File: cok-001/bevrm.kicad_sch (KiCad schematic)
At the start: 11 parts, among them U6103 NCP5318FTR2G, U6104 iP2003APbF, U6105 iP2003APbF, U6106 iP2003APbF, U6107 TC7SG08FU

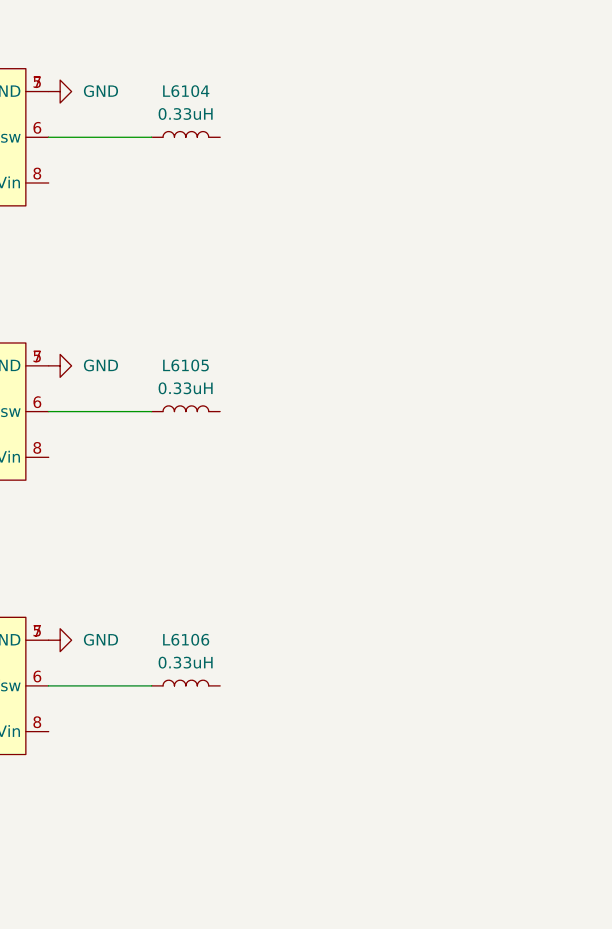
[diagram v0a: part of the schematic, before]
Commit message: chris proad
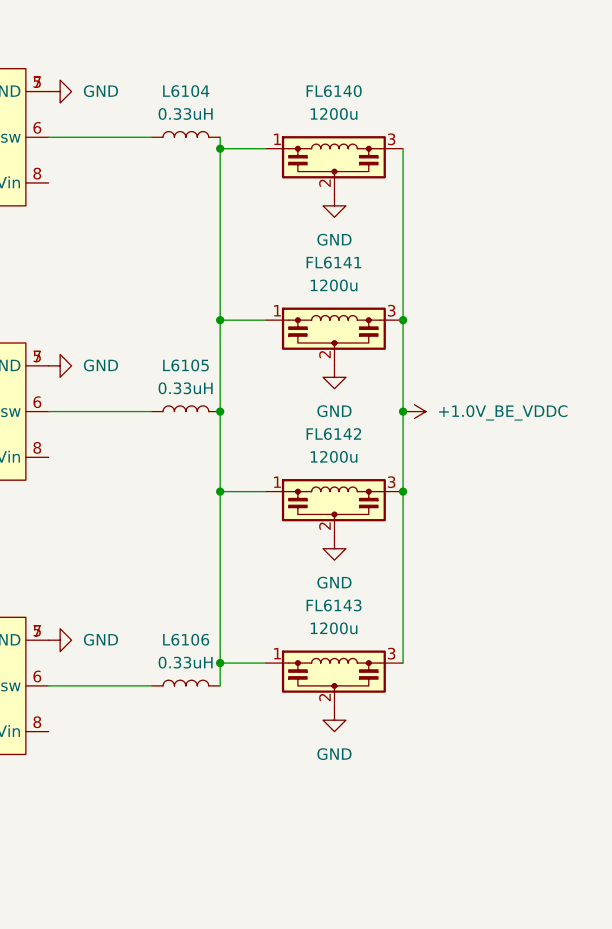
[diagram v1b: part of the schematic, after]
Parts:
- added FL6140, FL6141, FL6142, FL6143: 1200u, PS3:Proadlizer, symbol Device:Filter_EMI_CLC
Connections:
- net GND: now also FL6140.2, FL6141.2, FL6142.2, FL6143.2
- net at L6105.2: now also L6104.2, L6106.2, FL6140.1, FL6141.1, FL6142.1, FL6143.1
- new net +1.0V_BE_VDDC: FL6140.3, FL6141.3, FL6142.3, FL6143.3

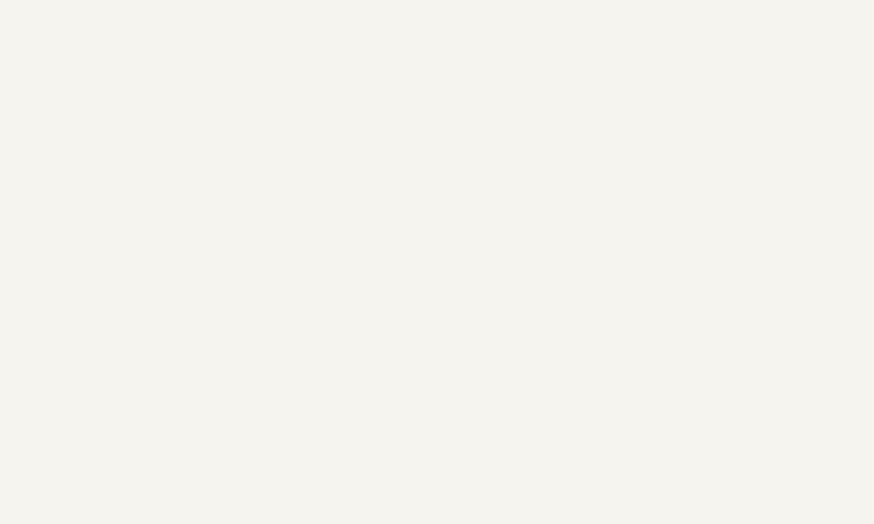
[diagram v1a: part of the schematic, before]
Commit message: temp sensor and clock
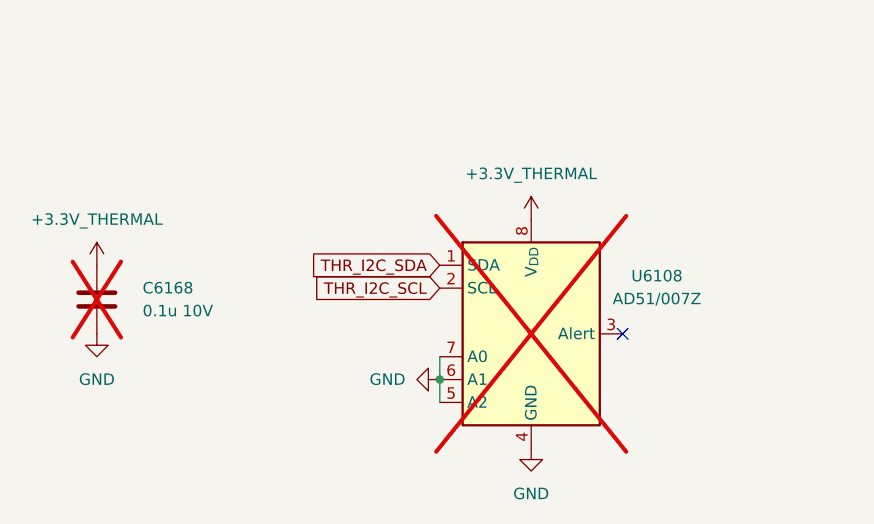
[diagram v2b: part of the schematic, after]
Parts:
- added C6168: 0.1u 10V, Capacitor_SMD:C_0402_1005Metric, symbol Device:C
- added U6108: AD51/007Z, Package_SO:MSOP-8_3x3mm_P0.65mm, symbol Sensor_Temperature:MCP9804_MSOP
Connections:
- net GND: now also C6168.2, U6108.4 (GND), U6108.5 (A2), U6108.6 (A1), U6108.7 (A0)
- new net +3.3V_THERMAL: C6168.1, U6108.8 (V_{DD})
- new net THR_I2C_SCL: U6108.2 (SCL)
- new net THR_I2C_SDA: U6108.1 (SDA)
- no-connect marks 0 -> 1

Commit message: msop
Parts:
- U6108: footprint Package_SO:MSOP-8_3x3mm_P0.65mm -> PS3:MSOP-8_2.9x4mm_P0.65mm
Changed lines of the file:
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@@
 			)
 		)
-		(property "Footprint" "Package_SO:MSOP-8_3x3mm_P0.65mm"
+		(property "Footprint" "PS3:MSOP-8_2.9x4mm_P0.65mm"
 			(at 43.18 176.53 0)
 			(effects

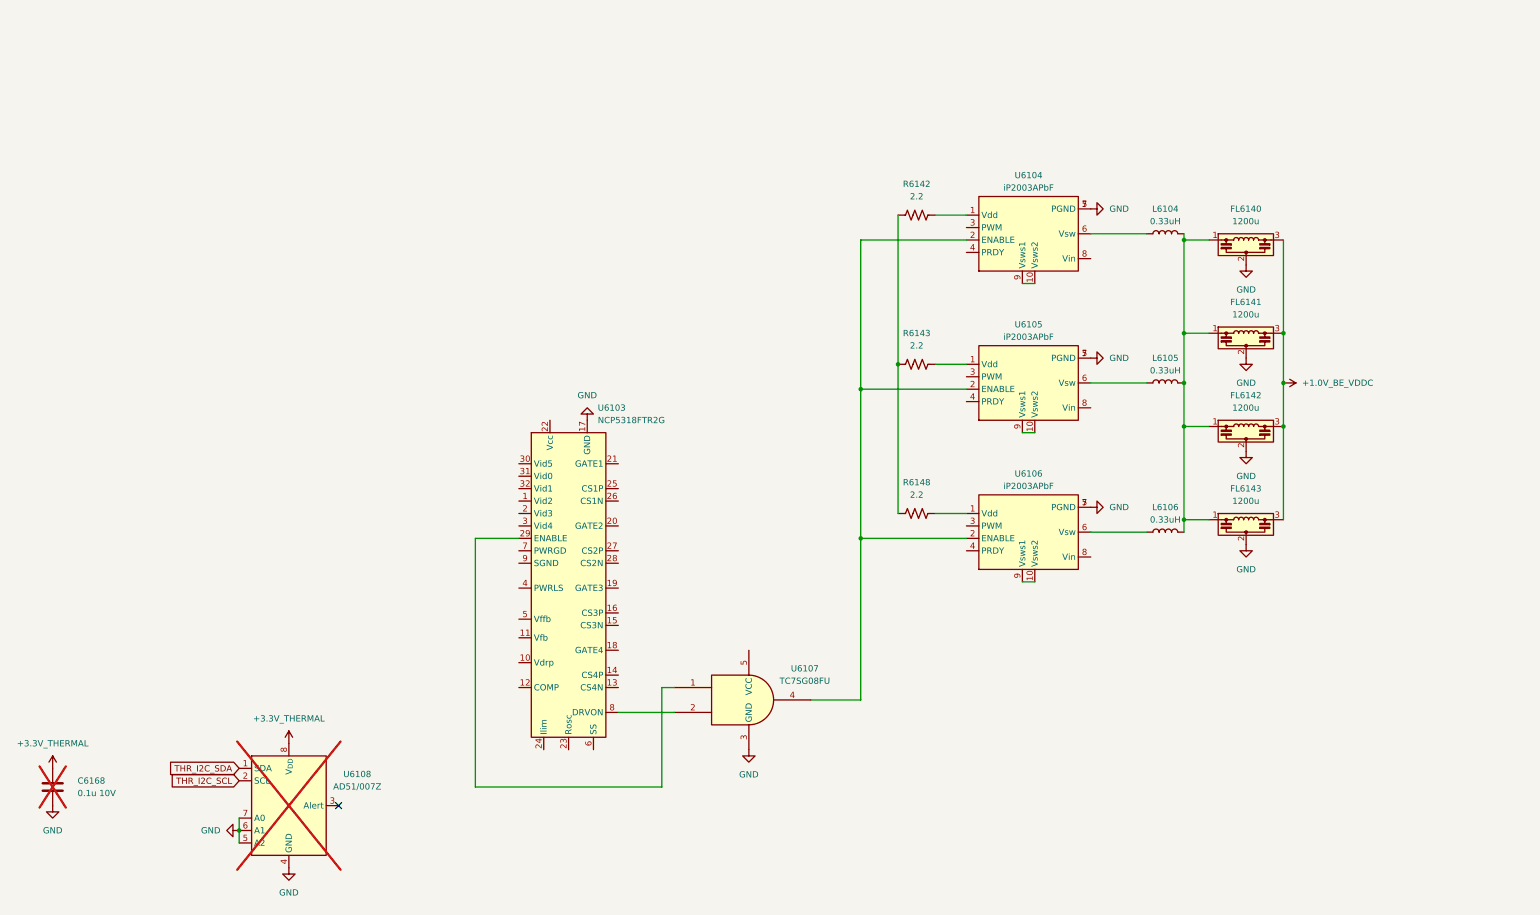
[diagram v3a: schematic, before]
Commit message: current sense
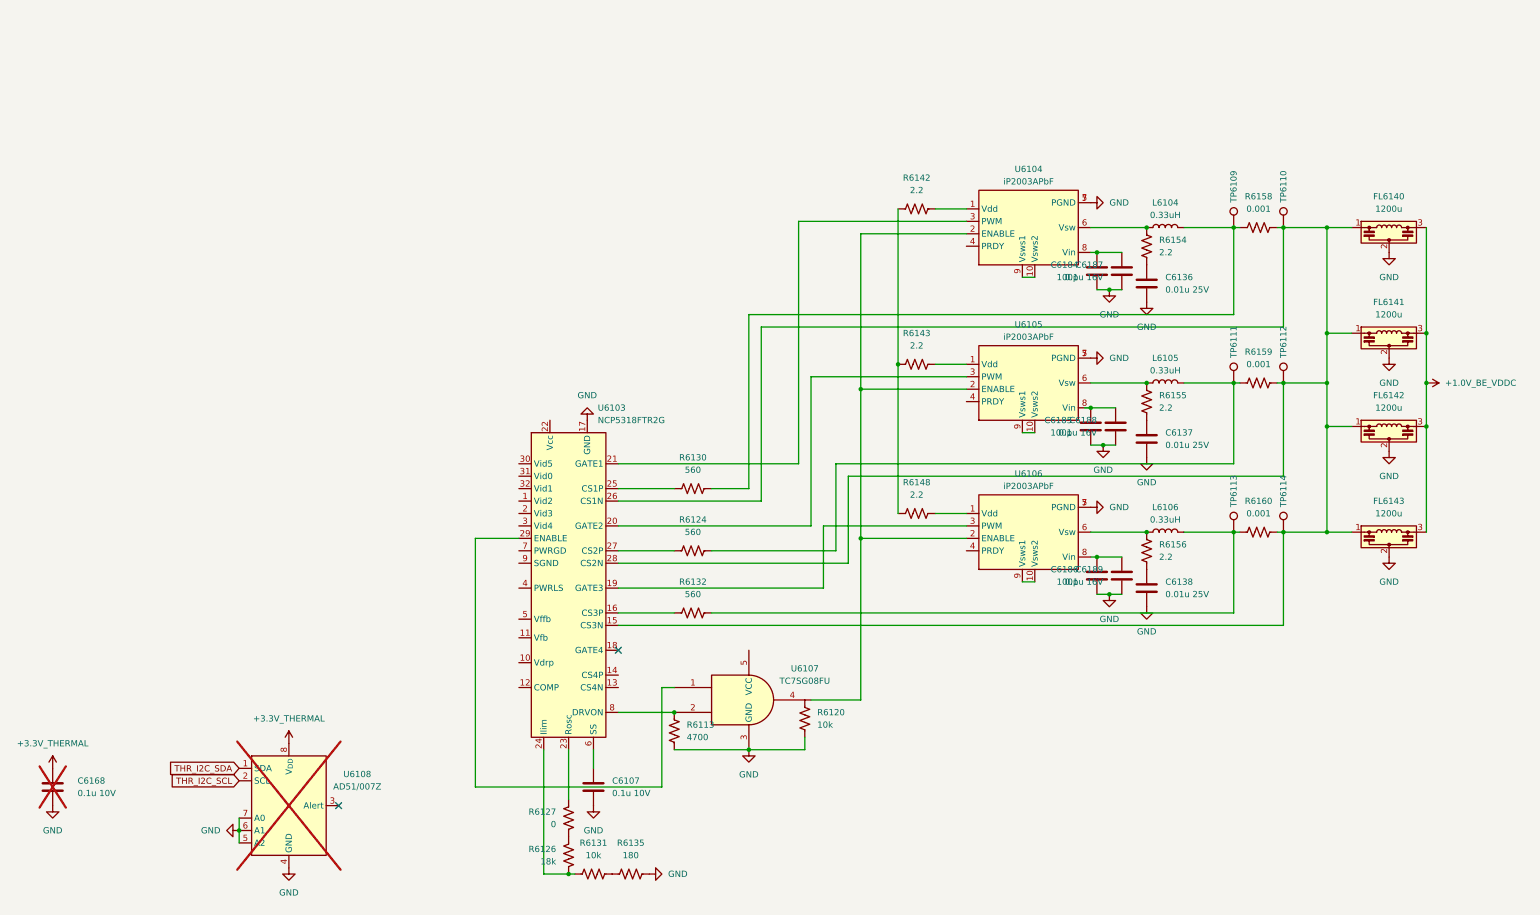
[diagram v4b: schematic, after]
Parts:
- added C6107: 0.1u 10V, Capacitor_SMD:C_0402_1005Metric, symbol Device:C
- added C6136, C6137, C6138: 0.01u 25V, Capacitor_SMD:C_0402_1005Metric, symbol Device:C
- added C6184, C6185, C6186: 100p, Capacitor_SMD:C_0402_1005Metric, symbol Device:C
- added C6187, C6188, C6189: 0.1u 16V, Capacitor_SMD:C_0402_1005Metric, symbol Device:C
- added R6113: 4700, Resistor_SMD:R_0402_1005Metric, symbol Device:R_US
- added R6120, R6131: 10k, Resistor_SMD:R_0402_1005Metric, symbol Device:R_US
- added R6124, R6130, R6132: 560, Resistor_SMD:R_0402_1005Metric, symbol Device:R_US
- added R6126: 18k, Resistor_SMD:R_0402_1005Metric, symbol Device:R_US
- added R6127: 0, Resistor_SMD:R_0402_1005Metric, symbol Device:R_US
- added R6135: 180, Resistor_SMD:R_0402_1005Metric, symbol Device:R_US
- added R6154, R6155, R6156: 2.2, Resistor_SMD:R_0805_2012Metric, symbol Device:R_US
- added R6158, R6159, R6160: 0.001, Resistor_SMD:R_2512_6332Metric, symbol Device:R_US
- added TP6109, TP6110, TP6111, TP6112, TP6113, TP6114: TestPoint, TestPoint:TestPoint_Pad_D1.5mm, symbol Connector:TestPoint
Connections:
- net GND: now also C6107.1, C6136.1, C6137.1, C6138.1, C6184.1, C6185.1, C6186.1, C6187.1, C6188.1, C6189.1, R6113.1, R6120.1, R6135.2
- net at L6105.1: now also R6124.2, R6159.1, TP6111.1; no longer U6105.6 (Vsw)
- net at FL6140.1, FL6141.1, FL6142.1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: now also U6103.15 (CS3N), U6103.26 (CS1N), U6103.28 (CS2N), R6158.2, R6159.2, R6160.2, TP6110.1, TP6112.1, TP6114.1; no longer L6104.2, L6105.2, L6106.2
- net at U6106.3 (PWM): now also U6103.19 (GATE3)
- net at U6106.6 (Vsw): now also L6106.2, R6156.2; no longer L6106.1
- net at U6106.8 (Vin): now also C6186.2, C6189.2
- net at U6105.3 (PWM): now also U6103.20 (GATE2)
- net at U6105.8 (Vin): now also C6185.2, C6188.2
- net at U6103.8 (DRVON), U6107.2: now also R6113.2
- net at U6104.3 (PWM): now also U6103.21 (GATE1)
- net at U6104.6 (Vsw): now also L6104.2, R6154.2; no longer L6104.1
- net at U6104.8 (Vin): now also C6184.2, C6187.2
- net at U6103.16 (CS3P): now also R6132.1
- net at U6103.23 (Rosc): now also R6127.2
- net at U6103.24 (Ilim): now also R6126.1, R6131.1
- net at U6103.25 (CS1P): now also R6130.1
- net at U6103.27 (CS2P): now also R6124.1
- net at U6103.6 (SS): now also C6107.2
- new net: L6105.2, R6155.2, U6105.6 (Vsw)
- new net: C6137.2, R6155.1
- new net: C6136.2, R6154.1
- new net: L6104.1, R6130.2, R6158.1, TP6109.1
- new net: C6138.2, R6156.1
- new net: R6131.2, R6135.1
- new net: L6106.1, R6132.2, R6160.1, TP6113.1
- new net: R6126.2, R6127.1
- no-connect marks 1 -> 2
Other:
- moved on the sheet: FL6140, FL6141, FL6142, FL6143, L6104, L6105, L6106, R6142, U6104

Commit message: pid in
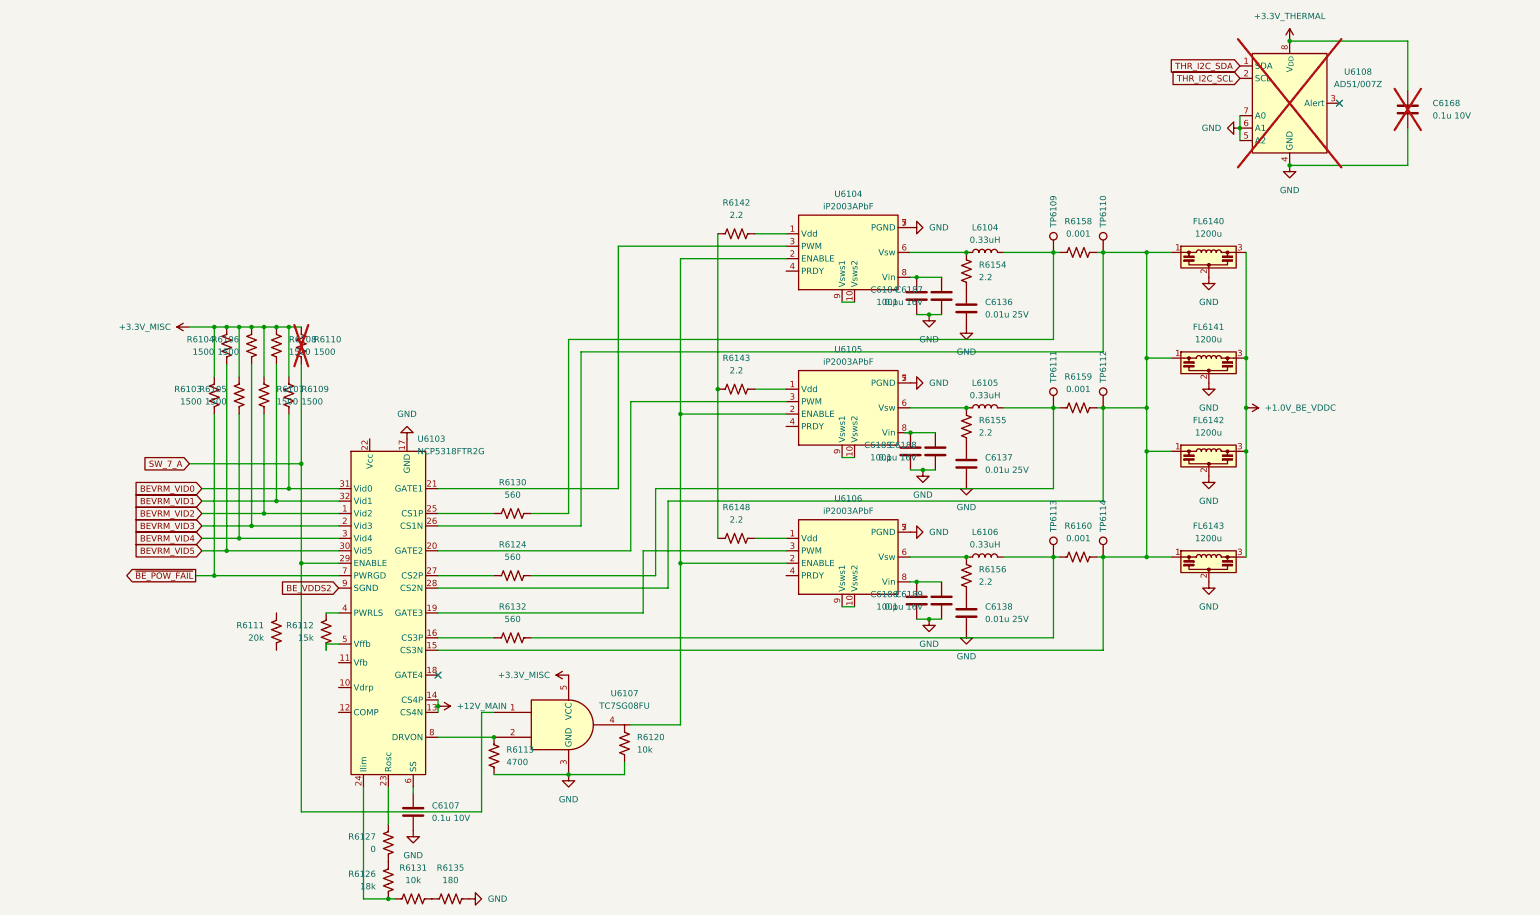
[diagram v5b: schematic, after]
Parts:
- added R6103, R6104, R6105, R6106, R6107, R6108, R6109, R6110: 1500, Resistor_SMD:R_0402_1005Metric, symbol Device:R_US
- added R6111: 20k, Resistor_SMD:R_0402_1005Metric, symbol Device:R_US
- added R6112: 15k, Resistor_SMD:R_0402_1005Metric, symbol Device:R_US
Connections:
- net SW_7_A: now reaches U6103.29 (ENABLE), U6107.1
- net SW_7_A: now also R6110.1
- net +3.3V_MISC: now reaches U6107.5 (VCC)
- net +3.3V_MISC: now also R6103.2, R6104.2, R6105.2, R6106.2, R6107.2, R6108.2, R6109.2, R6110.2
- net BEVRM_VID2: now reaches U6103.1 (Vid2)
- net BEVRM_VID2: now also R6107.1
- net +12V_MAIN: now reaches U6103.13 (CS4N)
- net +12V_MAIN: now also U6103.14 (CS4P)
- net BEVRM_VID3: now reaches U6103.2 (Vid3)
- net BEVRM_VID3: now also R6106.1
- net BEVRM_VID4: now reaches U6103.3 (Vid4)
- net BEVRM_VID4: now also R6105.1
- net BEVRM_VID5: now reaches U6103.30 (Vid5)
- net BEVRM_VID5: now also R6104.1
- net BEVRM_VID0: now reaches U6103.31 (Vid0)
- net BEVRM_VID0: now also R6109.1
- net BEVRM_VID1: now reaches U6103.32 (Vid1)
- net BEVRM_VID1: now also R6108.1
- net at U6103.4 (PWRLS): now also R6112.2
- net at U6103.5 (Vffb): now also R6112.1
- net ~{BE_POW_FAIL}: now reaches U6103.7 (PWRGD)
- net ~{BE_POW_FAIL}: now also R6103.1
- net BE_VDDS2: now reaches U6103.9 (SGND)
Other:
- moved on the sheet: C6107, C6136, C6137, C6138, C6168, C6184, C6185, C6186, C6187, C6188, C6189, FL6140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
